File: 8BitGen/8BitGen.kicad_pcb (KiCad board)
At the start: 2 copper layers, 90.4 x 50.5 mm, 12 parts, among them J1 Input Header, J2 Thru Hole Pads, J3 TRS, U1 74HC595, U2 SN7404N, U3 LM358, U4 YM3812, U5 YM3014B, X1 SG-531

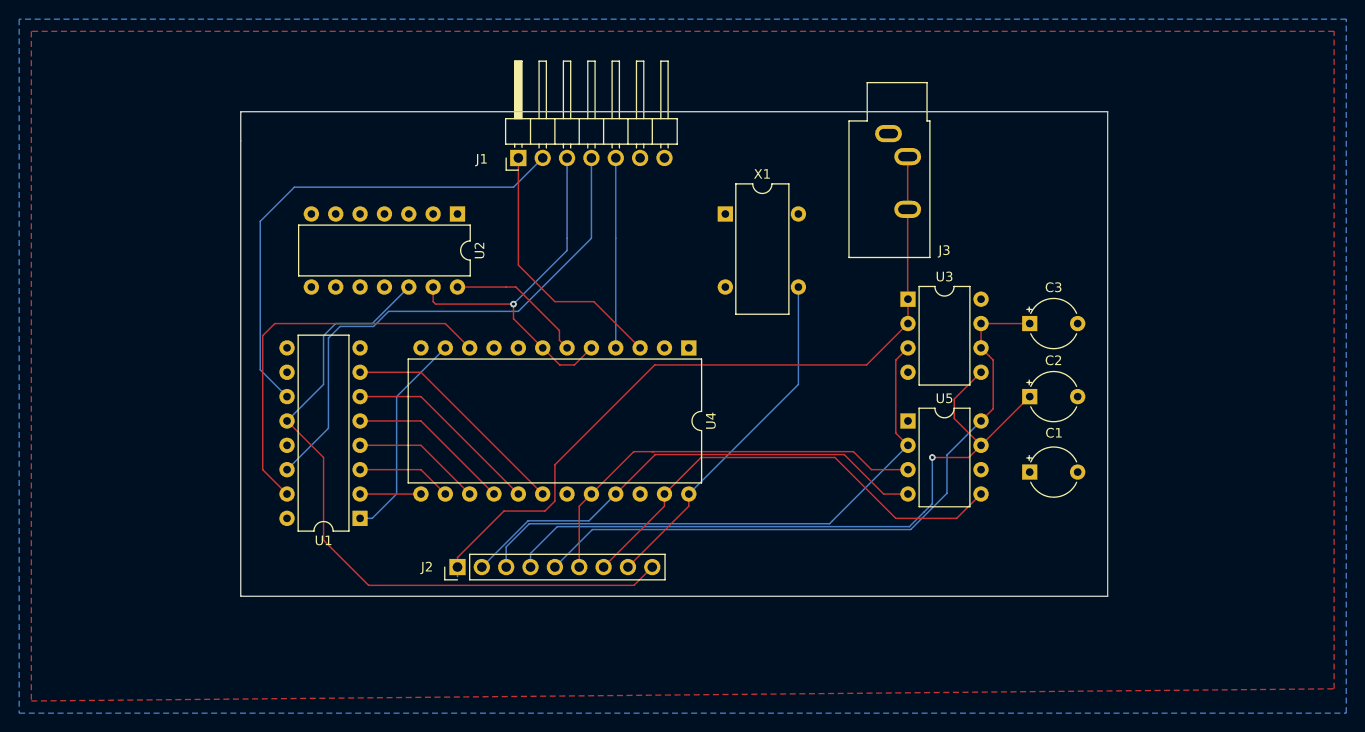
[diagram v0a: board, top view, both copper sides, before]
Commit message: Add track file
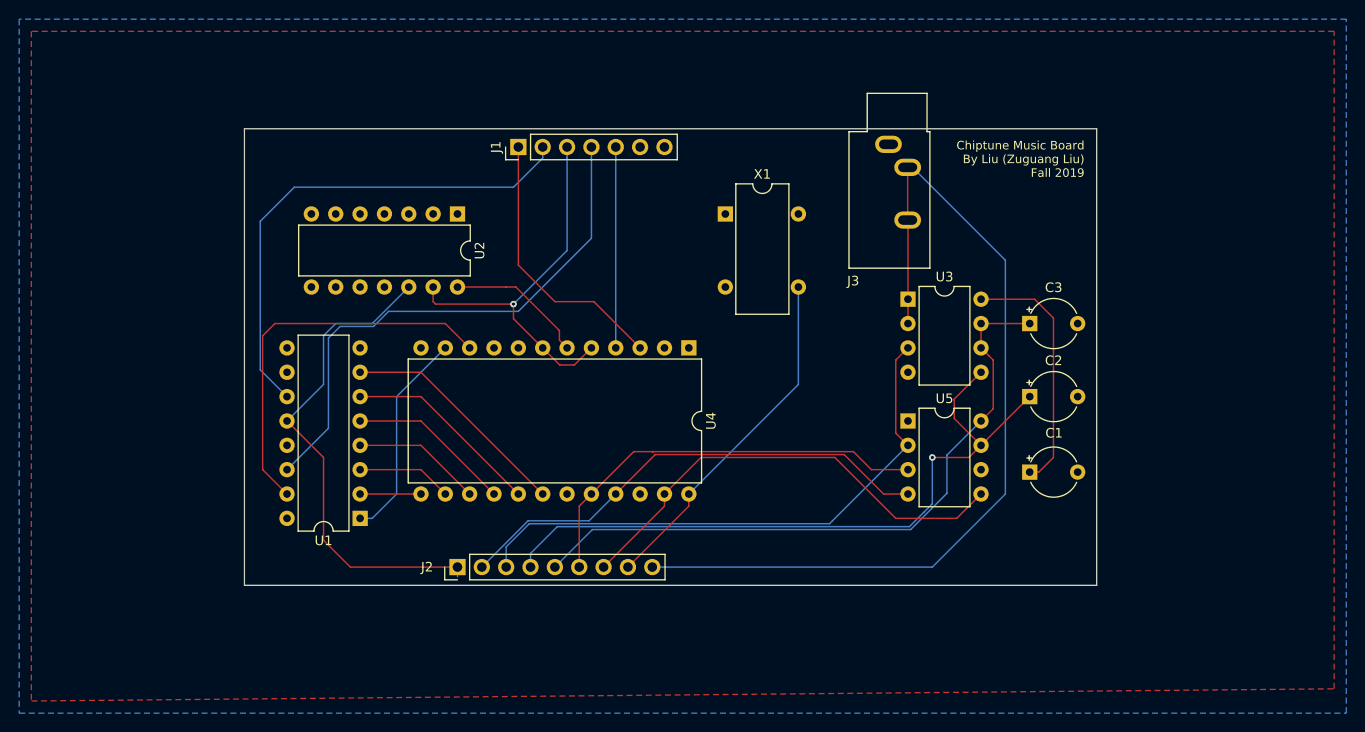
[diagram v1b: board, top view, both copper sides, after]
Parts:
- J1: footprint Connector_PinHeader_2.54mm:PinHeader_1x07_P2.54mm_Horizontal -> Connector_PinHeader_2.54mm:PinHeader_1x07_P2.54mm_Vertical
- moved J1 1.14 mm to (86.4, 33.7)
- moved J3 1.12 mm to (125.0, 33.4)
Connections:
- J2 pad 1: AUDIO_LINE -> REG_CLK
- J2 pad 9: REG_CLK -> AUDIO_LINE
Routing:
- net +5V: track 14.7 -> 40.7 mm
- net REG_CLK: track 72.5 -> 51.6 mm
- net AUDIO_LINE: track 78.7 -> 94.9 mm
- net YM_RST_N: track 27.5 -> 28.6 mm
- net YM_A0: track 19.8 -> 21.0 mm
- net WR_N: track 40.0 -> 41.1 mm
- net SERIAL_IN: track 55.6 -> 56.8 mm
- net SERIAL_CLK: track 51.6 -> 52.8 mm
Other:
- board size 90.4 x 50.5 mm -> 88.9 x 47.6 mm
- board text added: "Chiptune Music Board By Liu (Zuguang Liu) Fall 2019"
